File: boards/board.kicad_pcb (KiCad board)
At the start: 2 copper layers, 118 x 70 mm, 61 parts, among them J1 Conn_01x02, J2 Conn_01x02, J3 Conn_01x03, J4 Conn_01x06, J5 Conn_01x05, J6 Conn_01x02, J7 Conn_02x03_Odd_Even, J8 Conn_02x05_Odd_Even, Q1 2N2907, Q2 2n2222, Q3 IRF4905, Q4 2N7000, SW1 Switch, U1 ESP32-WROOM-32U, U2 LM393, U3 LM7805_TO220, U4 LM1117DT-ADJ, U5 LM1117DT-ADJ

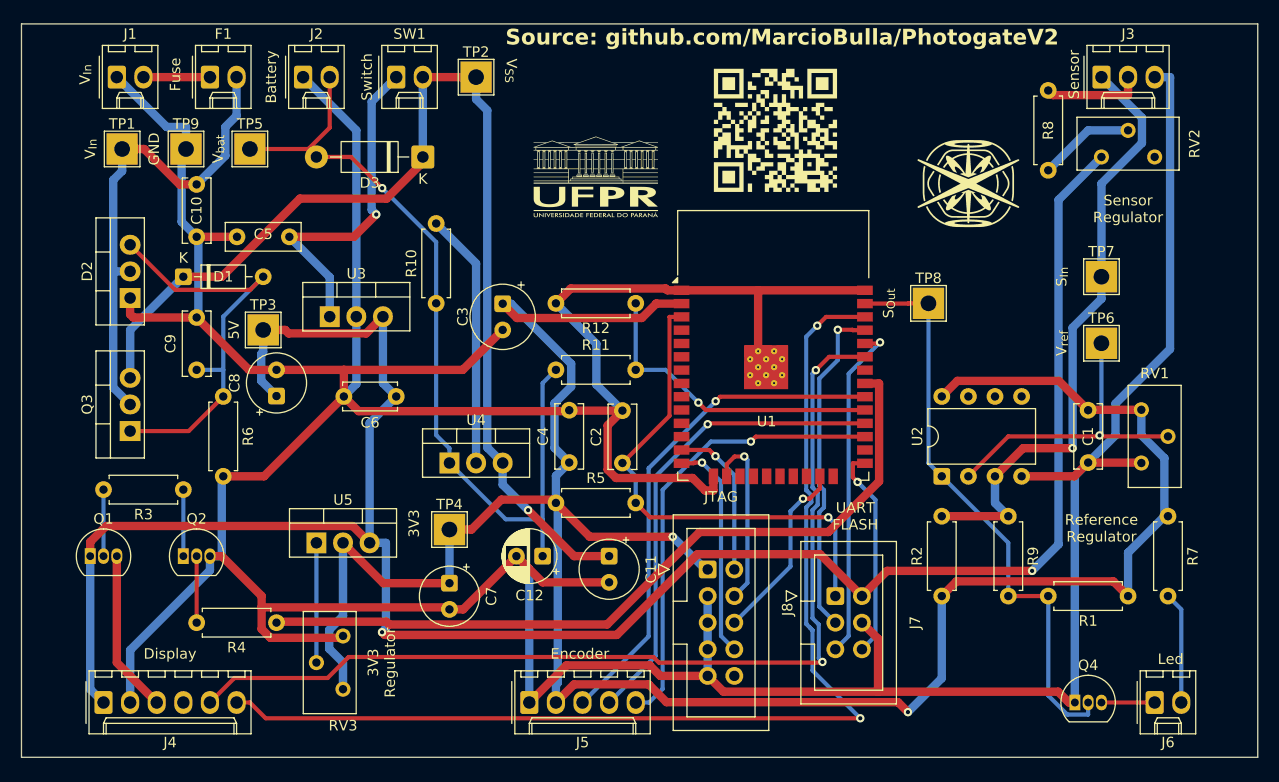
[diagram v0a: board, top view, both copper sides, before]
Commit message: update PCB and create gerber
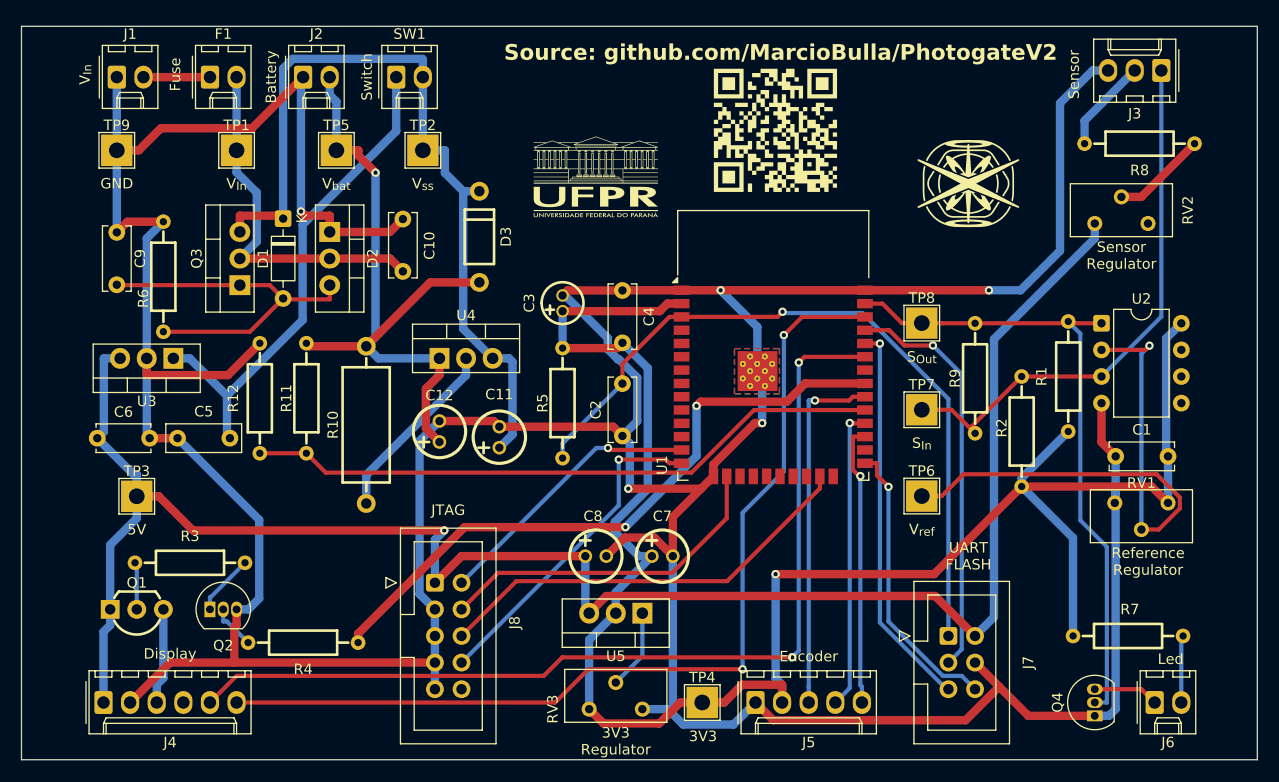
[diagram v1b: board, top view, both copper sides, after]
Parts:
- C11, C7, C8: footprint Capacitor_THT:CP_Radial_Tantal_D5.5mm_P2.50mm -> easyeda2kicad:CAP-TH_BD5.0-P2.00-D0.8-FD
- C12: footprint Capacitor_THT:CP_Radial_D5.0mm_P2.50mm -> easyeda2kicad:CAP-TH_BD5.0-P2.00-D0.8-FD
- C3: footprint Capacitor_THT:CP_Radial_Tantal_D6.0mm_P2.50mm -> easyeda2kicad:CAP-TH_BD4.0-P1.50-D0.8-FD
- D3: footprint Diode_THT:D_DO-41_SOD81_P10.16mm_Horizontal -> easyeda2kicad:DO-41_BD2.4-L4.7-P8.70-D0.9-RD
- Q1: footprint Package_TO_SOT_THT:TO-92_Inline -> easyeda2kicad:TO-92-3_L4.8-W3.7-P2.54-R
- QRcode git: value LOGO -> LOGO3
- R1, R11, R12, R2, R3, R4, R5, R6, R7, R8: footprint Resistor_THT:R_Axial_DIN0207_L6.3mm_D2.5mm_P7.62mm_Horizontal -> easyeda2kicad:RES-TH_BD2.3-L6.5-P10.50-D0.5
- R10: footprint Resistor_THT:R_Axial_DIN0207_L6.3mm_D2.5mm_P7.62mm_Horizontal -> easyeda2kicad:RES-TH_BD4.5-L11.0-P15.00-D0.7
- R9: value 50k -> 51k; footprint Resistor_THT:R_Axial_DIN0207_L6.3mm_D2.5mm_P7.62mm_Horizontal -> easyeda2kicad:RES-TH_BD2.3-L6.5-P10.50-D0.5
- U1: value ESP32-WROOM-32U -> ESP32-WROOM-32D; footprint RF_Module:ESP32-WROOM-32 -> RF_Module:ESP32-WROOM-32D
- moved R12 37.0 mm to (117.8, 100.5), turned to 90 degrees
- moved C8 34.1 mm to (149.9, 115.6), turned to 0 degrees
- moved U5 31.8 mm to (154.3, 121.0), turned to 180 degrees
- moved TP4 29.2 mm to (160.0, 129.5)
- moved C6 28.8 mm to (102.3, 104.3), turned to 0 degrees
- moved J8 26.1 mm to (134.5, 118.1)
- moved R11 24.0 mm to (122.2, 100.5), turned to -90 degrees
- moved RV3 23.6 mm to (149.2, 130.2), turned to 90 degrees
- moved TP6 22.5 mm to (181.0, 109.8)
- moved R1 21.7 mm to (194.9, 98.4), turned to 90 degrees
- moved J5 21.6 mm to (165.1, 129.5)
- moved C10 21.4 mm to (131.4, 88.4), turned to 90 degrees
- moved TP7 21.3 mm to (181.0, 101.6)
- moved U2 21.1 mm to (198.1, 93.3), turned to 0 degrees
- moved C7 20.5 mm to (156.2, 115.6), turned to 0 degrees
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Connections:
- J8 pad 1: +3V3 -> +5V
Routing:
- net +3V3: track 230.0 -> 180.5 mm, vias 2 -> 1
- net GND: track 480.3 -> 438.3 mm, vias 0 -> 5
- net /V_bat: track 29.8 -> 61.0 mm, vias 1 -> 0
- net +5V: track 206.7 -> 178.0 mm, vias 2 -> 1
- net VSS: track 105.3 -> 78.7 mm, vias 1 -> 0
- net Net-(U2A--): track 29.6 -> 54.6 mm
- net /TDO: track 17.7 -> 41.2 mm, vias 1 -> 0
- net /EN: track 48.0 -> 70.6 mm
- net /DT: track 45.5 -> 28.7 mm
- net /CLK: track 43.5 -> 27.0 mm
- net /TCK: track 17.1 -> 32.9 mm, vias 1 -> 0
- net Net-(D3-A): track 80.2 -> 64.8 mm
- net VDC: track 32.6 -> 47.9 mm, vias 1 -> 0
- net /SCL: track 105.9 -> 91.6 mm
- net /SW: track 48.4 -> 34.9 mm
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- added copper zone on B.Cu, net GND
- added copper zone on F.Cu, net GND
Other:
- board text added: "V_{ss}"
- board text removed: "V_{SS}"
